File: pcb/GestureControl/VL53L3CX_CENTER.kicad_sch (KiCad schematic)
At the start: 67 parts, among them J13 690367291076, J14 690367291076, J15 690367291076, J16 690367291076, J20 690367291076, J21 690367291076, J22 690367291076, J23 690367291076, U3 VL53L3CXV0DH_1, U4 VL53L3CXV0DH_1, U5 VL53L3CXV0DH_1, U8 VL53L3CXV0DH_1, U9 VL53L3CXV0DH_1

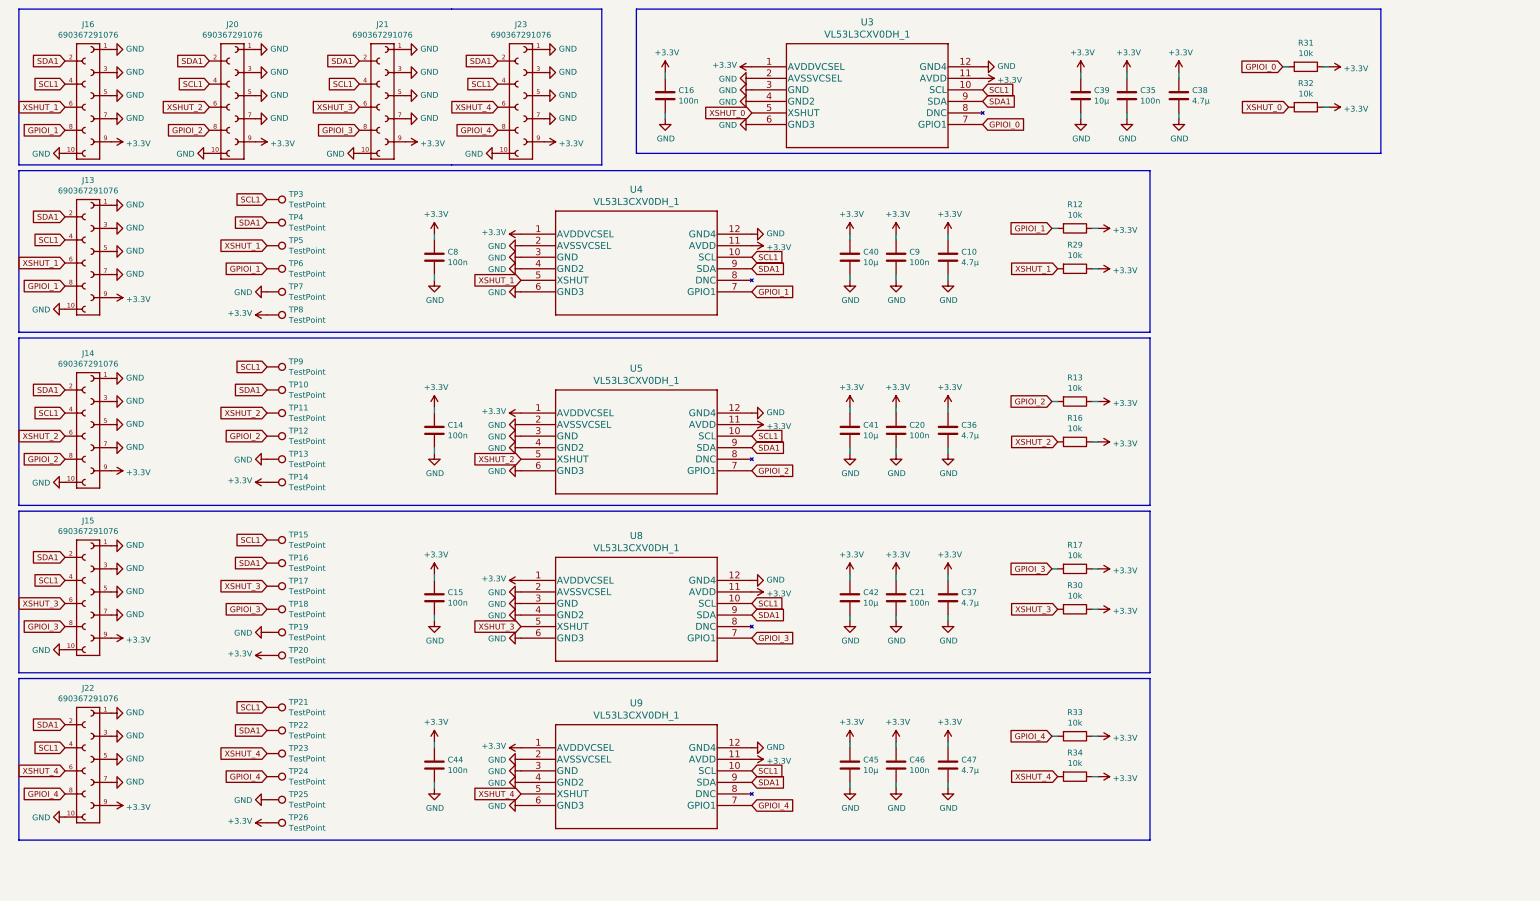
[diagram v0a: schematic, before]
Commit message: edit PCB + add docs
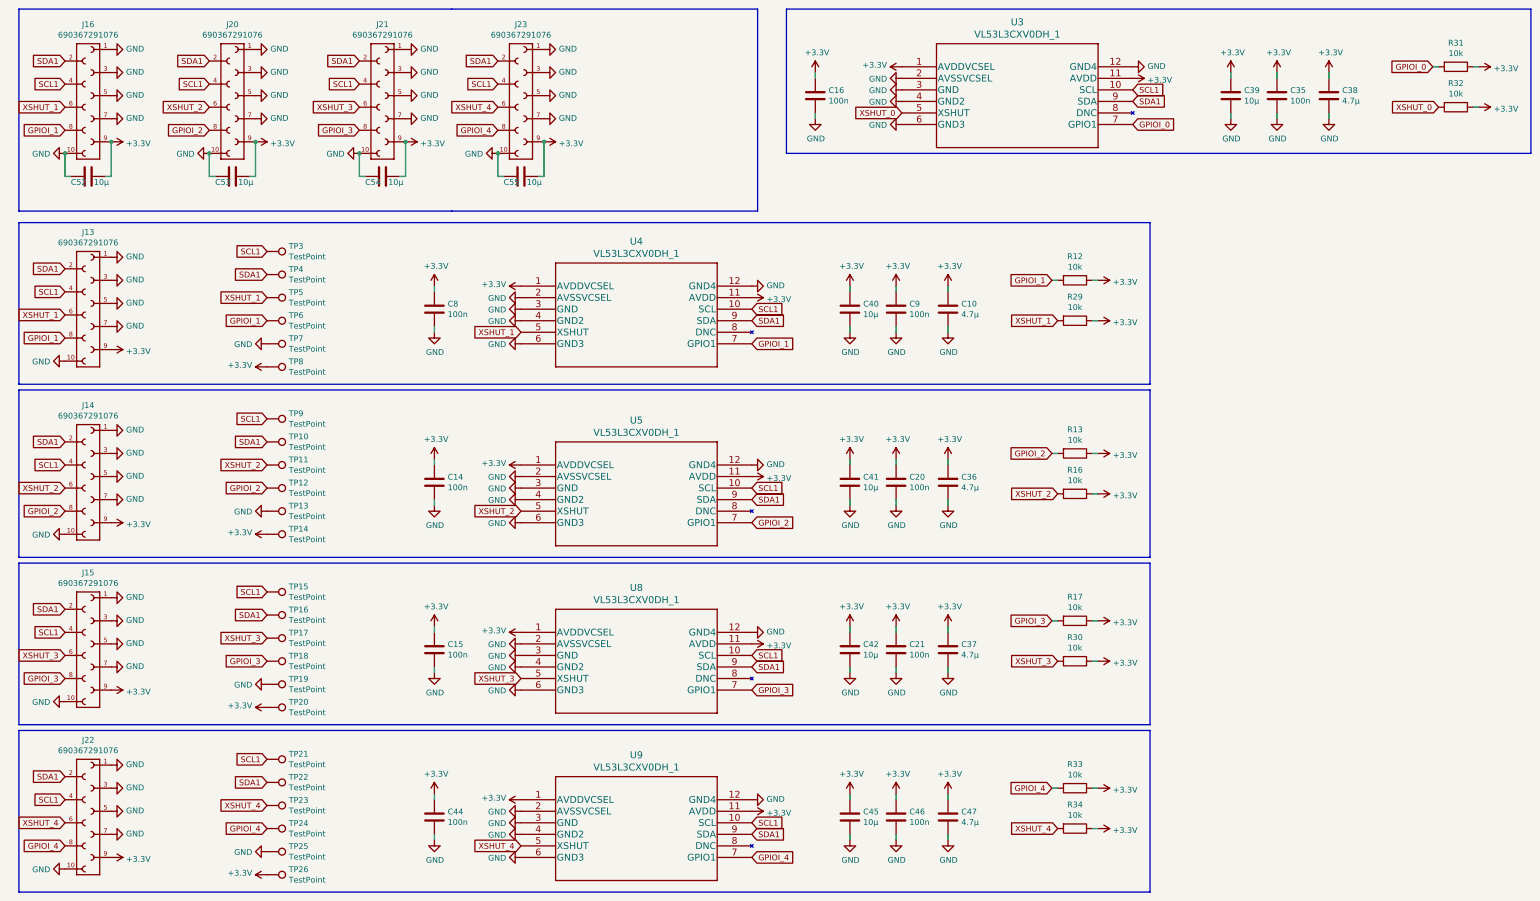
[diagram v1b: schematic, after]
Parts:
- added C52, C53, C54, C55: 10µ, Capacitor_SMD:C_1206_3216Metric_Pad1.33x1.80mm_HandSolder, symbol Device:C
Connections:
- net +3V3: now also C52.1, C53.1, C54.1, C55.1
- net GND: now also C52.2, C53.2, C54.2, C55.2
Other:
- moved on the sheet: C10, C14, C15, C16, C20, C21, C35, C36, C37, C38, C39, C40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
